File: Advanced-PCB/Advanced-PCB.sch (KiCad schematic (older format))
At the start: 150 parts, among them J1 USB_mini_micro_B, SW1 Esc, SW10 Win 1.25, SW11 2, SW12 W, SW13 S, SW14 X, SW15 Alt 1.25, SW16 3, SW17 E, SW18 D, SW19 C, SW2 Tab 1.50, SW20 4, SW21 R, SW22 F, SW23 V, SW24 5, SW25 T, SW26 G, SW27 B, SW28 Space 6.25, SW29 6, SW3 Caps 1.75, SW30 Y, SW31 H, SW32 N, SW33 7, SW34 U, SW35 J, SW36 M, SW37 8, SW38 I, SW39 K, SW4 Shift 2.25, SW40 ,, SW41 9, SW42 O, SW43 L, SW44 ., SW45 Alt 1.25, SW46 0, SW47 P, SW48 ;, SW49 /, SW5 Ctrl 1.25, SW50 Fn 1.25, SW51 -, SW52 [, SW53 ', SW54 Shift 1.75, SW55 Left Arrow, SW56 =, SW57 ], SW58 Enter 2.25, SW59 Up Arrow, SW6 1, SW60 Down Arrow, SW61 Back 2.00, SW62 \\ 1.50, SW63 Pg Up, SW64 Pg Down, SW65 Right Arrow, SW66 `, SW67 Del, SW7 Q, SW8 A, SW9 Z, U1 ATMEGA32U4, X1 16MHz

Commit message: Alternate Row 0
Alternate Row zero with 1u right side keys added.
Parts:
- added D? (x3): 1N4148W, Diode_SMD:D_SOD-123, symbol Device:D_Small
- added SW?: Fn 1.00, acheron_MXH:MX125H, symbol acheronSymbols:MXSwitch
- added SW?: Alt 1.00, acheron_MXH:MX125H, symbol acheronSymbols:MXSwitch
- added SW?: Ctrl 1.00, acheron_MXH:MX125H, symbol acheronSymbols:MXSwitch
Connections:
- wire segments 305 -> 315
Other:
- note added: "BOTTOM LAYOUT 1\n"
- note added: "BOTTOM LAYOUT 2\n\n"

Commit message: Layout Simplified
Layout Simplified by stacking switches unable to be used at same time because of different kb layouts. Right alt and fn with ctrl left down as seperate row.
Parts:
- removed D? (x2): 1N4148W, Diode_SMD:D_SOD-123, symbol Device:D_Small
- J1: symbol keyboard_parts:USB_mini_micro_B -> Advanced-PCB-rescue:USB_mini_micro_B-keyboard_parts
- SW1, SW10, SW11, SW12, SW13, SW14, SW15, SW16, SW17, SW18, SW19, SW2, SW20, SW21, SW22, SW23, SW24, SW25, SW26, SW27, SW28, SW29, SW3, SW30, SW31, SW32, SW33, SW34, SW35, SW36, SW37, SW38, SW39, SW4, SW40, SW41, SW42, SW43, SW44, SW45, SW46, SW47, SW48, SW49, SW5, SW50, SW51, SW52, SW53, SW54, SW55, SW56, SW57, SW58, SW59, SW6, SW60, SW61, SW62, SW63, SW64, SW65, SW66, SW67, SW7, SW8, SW9: symbol acheronSymbols:MXSwitch -> Advanced-PCB-rescue:MXSwitch-acheronSymbols
- SW68, SW69, SW70: renamed from SW?; footprint acheron_MXH:MX125H -> acheron_MXH:MX100H; symbol acheronSymbols:MXSwitch -> Advanced-PCB-rescue:MXSwitch-acheronSymbols
- SWPw1: symbol keyboard_parts:SW_PUSH -> Advanced-PCB-rescue:SW_PUSH-keyboard_parts
- U1: symbol keyboard_parts:ATMEGA32U4 -> Advanced-PCB-rescue:ATMEGA32U4-keyboard_parts
- X1: symbol keyboard_parts:XTAL_GND -> Advanced-PCB-rescue:XTAL_GND-keyboard_parts
- gave numbers to parts that had none: 1
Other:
- moved on the sheet: D70

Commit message: Rows And Columns Fixed
Fixed Issue to make all columns and rows linked properly
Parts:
- SW1, SW11, SW12, SW13, SW14, SW16, SW17, SW18, SW19, SW20, SW21, SW22, SW23, SW24, SW25, SW26, SW27, SW29, SW30, SW31, SW32, SW33, SW34, SW35, SW36, SW37, SW38, SW39, SW40, SW41, SW43, SW44, SW46, SW48, SW49, SW51, SW52, SW53, SW55, SW56, SW57, SW59, SW6, SW60, SW63, SW64, SW65, SW66, SW67, SW68, SW69, SW7, SW70, SW8, SW9: footprint acheron_MXH:MX100H -> acheron_MXA:MXA100
- SW10, SW15, SW45, SW5, SW50: footprint acheron_MXH:MX125H -> acheron_MXA:MXA125
- SW2, SW62: footprint acheron_MXH:MX150H -> acheron_MXA:MXA150
- SW28: footprint acheron_MXH:MX625HR -> acheron_MXA:MXA625R
- SW3, SW54: footprint acheron_MXH:MX175H -> acheron_MXA:MXA175
- SW4, SW58: footprint acheron_MXH:MX225HR -> acheron_MXA:MXA225R
- SW42: value O -> P; footprint acheron_MXH:MX100H -> acheron_MXA:MXA100
- SW47: value P -> O; footprint acheron_MXH:MX100H -> acheron_MXA:MXA100
- SW61: footprint acheron_MXH:MX200HR -> acheron_MXA:MXA200R
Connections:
- net Col1: now also U1.36 (PF7); no longer D1.1 (K), D10.1 (K), D11.1 (K), D12.1 (K), D13.1 (K), D14.1 (K), D15.1 (K), D16.1 (K), D17.1 (K), D18.1 (K), D19.1 (K), D2.1 (K), D20.1 (K), D21.1 (K), D22.1 (K), D23.1 (K), D24.1 (K), D25.1 (K), D26.1 (K), D27.1 (K), D28.1 (K), D29.1 (K), D3.1 (K), D30.1 (K), D31.1 (K), D32.1 (K), D33.1 (K), D34.1 (K), D35.1 (K), D36.1 (K), D37.1 (K), D38.1 (K), D39.1 (K), D4.1 (K), D40.1 (K), D41.1 (K), D42.1 (K), D43.1 (K), D44.1 (K), D45.1 (K), D46.1 (K), D47.1 (K), D48.1 (K), D49.1 (K), D5.1 (K), D50.1 (K), D51.1 (K), D52.1 (K), D53.1 (K), D54.1 (K), D55.1 (K), D56.1 (K), D57.1 (K), D58.1 (K), D59.1 (K), D6.1 (K), D60.1 (K), D61.1 (K), D62.1 (K), D63.1 (K), D64.1 (K), D65.1 (K), D66.1 (K), D67.1 (K), D7.1 (K), D70.1 (K), D8.1 (K), D9.1 (K), SW10.1 (Col), SW11.1 (Col), SW12.1 (Col), SW13.1 (Col), SW14.1 (Col), SW15.1 (Col), SW16.1 (Col), SW17.1 (Col), SW18.1 (Col), SW19.1 (Col), SW20.1 (Col), SW21.1 (Col), SW22.1 (Col), SW23.1 (Col), SW24.1 (Col), SW25.1 (Col), SW26.1 (Col), SW27.1 (Col), SW28.1 (Col), SW29.1 (Col), SW30.1 (Col), SW31.1 (Col), SW32.1 (Col), SW33.1 (Col), SW34.1 (Col), SW35.1 (Col), SW36.1 (Col), SW37.1 (Col), SW38.1 (Col), SW39.1 (Col), SW40.1 (Col), SW41.1 (Col), SW42.1 (Col), SW43.1 (Col), SW44.1 (Col), SW45.1 (Col), SW46.1 (Col), SW47.1 (Col), SW48.1 (Col), SW49.1 (Col), SW50.1 (Col), SW51.1 (Col), SW52.1 (Col), SW53.1 (Col), SW54.1 (Col), SW55.1 (Col), SW56.1 (Col), SW57.1 (Col), SW58.1 (Col), SW59.1 (Col), SW6.1 (Col), SW60.1 (Col), SW61.1 (Col), SW62.1 (Col), SW63.1 (Col), SW64.1 (Col), SW65.1 (Col), SW66.1 (Col), SW67.1 (Col), SW7.1 (Col), SW70.1 (Col), SW8.1 (Col), SW9.1 (Col), U1.38 (PF5), U1.39 (PF4), U1.40 (PF1), U1.41 (PF0)
- net Col10: now reaches U1.11 (PB3/MISO)
- net Col10: now also SW41.1 (Col), SW42.1 (Col), SW43.1 (Col), SW44.1 (Col), SW45.1 (Col), SW68.1 (Col)
- net Col11: now reaches U1.18 (PD0/INT0)
- net Col11: now also SW46.1 (Col), SW47.1 (Col), SW48.1 (Col), SW49.1 (Col), SW50.1 (Col), SW69.1 (Col)
- net Col12: now reaches U1.19 (PD1/INT1)
- net Col12: now also SW51.1 (Col), SW52.1 (Col), SW53.1 (Col), SW54.1 (Col), SW55.1 (Col), SW70.1 (Col)
- net Col13: now reaches U1.20 (PD2/RXD1)
- net Col13: now also SW56.1 (Col), SW57.1 (Col), SW58.1 (Col), SW59.1 (Col), SW60.1 (Col)
- net Col14: now reaches U1.21 (PD3/TXD1)
- net Col14: now also SW61.1 (Col), SW62.1 (Col), SW63.1 (Col), SW64.1 (Col), SW65.1 (Col)
- net Col15: now reaches U1.22 (PD5/XCK1)
- net Col15: now also SW66.1 (Col), SW67.1 (Col)
- net Col9: now reaches U1.25 (ICP1/PD4)
- net Col9: now also SW37.1 (Col), SW38.1 (Col), SW39.1 (Col), SW40.1 (Col)
- net Col8: now reaches U1.26 (T1/PD6)
- net Col8: now also SW33.1 (Col), SW34.1 (Col), SW35.1 (Col), SW36.1 (Col)
- net Col7: now reaches U1.27 (T0/PD7)
- net Col7: now also SW29.1 (Col), SW30.1 (Col), SW31.1 (Col), SW32.1 (Col)
- net Col6: now reaches U1.28 (PB4)
- net Col6: now also SW24.1 (Col), SW25.1 (Col), SW26.1 (Col), SW27.1 (Col), SW28.1 (Col)
- net Col5: now reaches U1.29 (PB5)
- net Col5: now also SW20.1 (Col), SW21.1 (Col), SW22.1 (Col), SW23.1 (Col)
- net Col4: now reaches U1.30 (PB6)
- net Col4: now also SW16.1 (Col), SW17.1 (Col), SW18.1 (Col), SW19.1 (Col)
- net Col3: now reaches U1.31 (PC6)
- net Col3: now also SW11.1 (Col), SW12.1 (Col), SW13.1 (Col), SW14.1 (Col), SW15.1 (Col)
- net Col2: now reaches U1.32 (PC7)
- net Col2: now also SW10.1 (Col), SW6.1 (Col), SW7.1 (Col), SW8.1 (Col), SW9.1 (Col)
- net Row4: now reaches U1.37 (PF6)
- net Row4: now also D1.1 (K), D11.1 (K), D16.1 (K), D20.1 (K), D24.1 (K), D29.1 (K), D33.1 (K), D37.1 (K), D41.1 (K), D46.1 (K), D51.1 (K), D56.1 (K), D6.1 (K), D61.1 (K), D66.1 (K)
- net at D45.2 (A), SW45.2 (Row): now also SW68.2 (Row)
- net at D50.2 (A), SW50.2 (Row): now also SW69.2 (Row)
- new net Row0: D10.1 (K), D15.1 (K), D28.1 (K), D45.1 (K), D5.1 (K), D50.1 (K), D55.1 (K), D60.1 (K), D65.1 (K), D70.1 (K), U1.41 (PF0)
- new net Row1: D14.1 (K), D19.1 (K), D23.1 (K), D27.1 (K), D32.1 (K), D36.1 (K), D4.1 (K), D40.1 (K), D44.1 (K), D49.1 (K), D54.1 (K), D59.1 (K), D64.1 (K), D9.1 (K), U1.40 (PF1)
- new net Row2: D13.1 (K), D18.1 (K), D22.1 (K), D26.1 (K), D3.1 (K), D31.1 (K), D35.1 (K), D39.1 (K), D43.1 (K), D48.1 (K), D53.1 (K), D58.1 (K), D63.1 (K), D8.1 (K), U1.39 (PF4)
- new net Row3: D12.1 (K), D17.1 (K), D2.1 (K), D21.1 (K), D25.1 (K), D30.1 (K), D34.1 (K), D38.1 (K), D42.1 (K), D47.1 (K), D52.1 (K), D57.1 (K), D62.1 (K), D67.1 (K), D7.1 (K), U1.38 (PF5)
- no-connect marks 22 -> 6
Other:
- moved on the sheet: D45, D50

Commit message: Mid Routing
In the Middle of Routing. All of tracing between initial components done. Switches still need to be traced and connected.
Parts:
- J1: symbol Advanced-PCB-rescue:USB_mini_micro_B-keyboard_parts -> Advanced-PCB-rescue:USB_mini_micro_B-keyboard_parts-Advanced-PCB-rescue
- SW1, SW10, SW11, SW12, SW13, SW14, SW15, SW16, SW17, SW18, SW19, SW2, SW20, SW21, SW22, SW23, SW24, SW25, SW26, SW27, SW28, SW29, SW3, SW30, SW31, SW32, SW33, SW34, SW35, SW36, SW37, SW38, SW39, SW4, SW40, SW41, SW42, SW43, SW44, SW45, SW46, SW47, SW48, SW49, SW5, SW50, SW51, SW52, SW53, SW54, SW55, SW56, SW57, SW58, SW59, SW6, SW60, SW61, SW62, SW63, SW64, SW65, SW66, SW67, SW68, SW69, SW7, SW70, SW8, SW9: symbol Advanced-PCB-rescue:MXSwitch-acheronSymbols -> Advanced-PCB-rescue:MXSwitch-acheronSymbols-Advanced-PCB-rescue
- SWPw1: symbol Advanced-PCB-rescue:SW_PUSH-keyboard_parts -> Advanced-PCB-rescue:SW_PUSH-keyboard_parts-Advanced-PCB-rescue
- U1: symbol Advanced-PCB-rescue:ATMEGA32U4-keyboard_parts -> Advanced-PCB-rescue:ATMEGA32U4-keyboard_parts-Advanced-PCB-rescue
- X1: value 16MHz -> XTAL_GND; footprint Crystal:Crystal_SMD_SeikoEpson_TSX3225-4Pin_3.2x2.5mm_HandSoldering -> kicad-library-master:crystal_FA238-TSX3225; symbol Advanced-PCB-rescue:XTAL_GND-keyboard_parts -> Advanced-PCB-rescue:XTAL_GND-keyboard_parts-Advanced-PCB-rescue
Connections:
- net +5V renamed GND

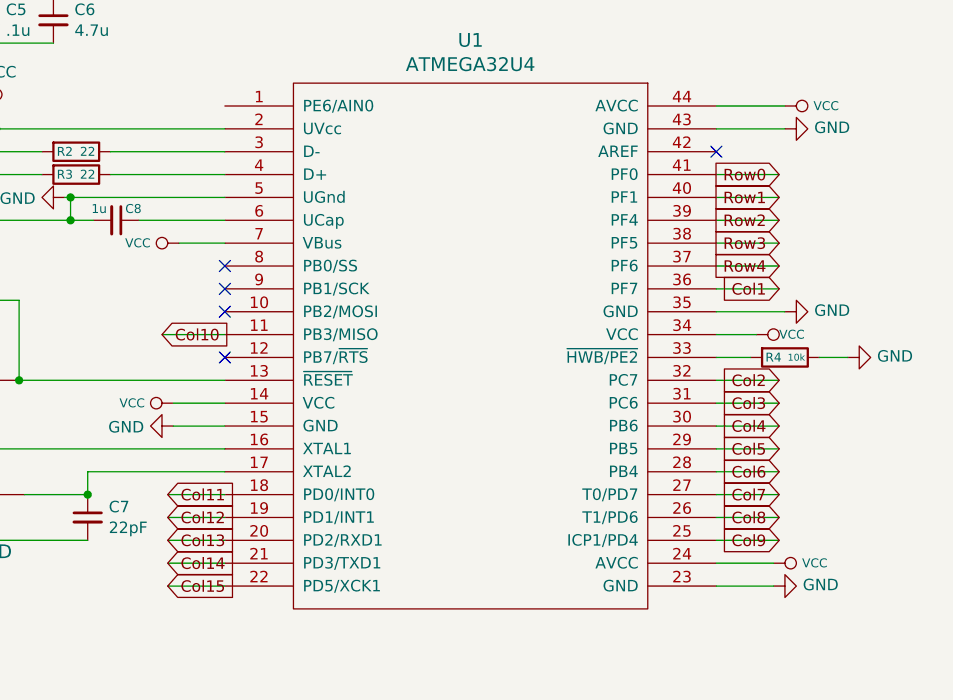
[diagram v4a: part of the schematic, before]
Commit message: Traces Continued
Continued Tracing All Rows and Half Columns completed.
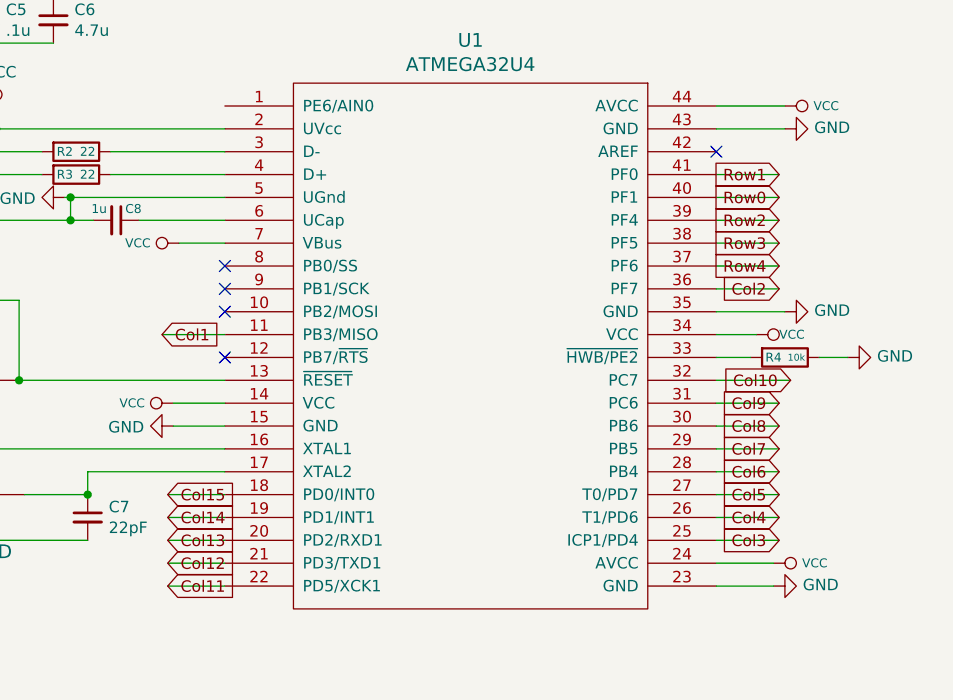
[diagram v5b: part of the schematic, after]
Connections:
- net Col1: now also U1.11 (PB3/MISO); no longer U1.36 (PF7)
- net Col10: now also U1.32 (PC7); no longer U1.11 (PB3/MISO)
- net Col11: now also U1.22 (PD5/XCK1); no longer U1.18 (PD0/INT0)
- net Col12: now also U1.21 (PD3/TXD1); no longer U1.19 (PD1/INT1)
- net Col14: now also U1.19 (PD1/INT1); no longer U1.21 (PD3/TXD1)
- net Col15: now also U1.18 (PD0/INT0); no longer U1.22 (PD5/XCK1)
- net Col2: now also U1.36 (PF7); no longer U1.32 (PC7)
- net Col3: now also U1.25 (ICP1/PD4); no longer U1.31 (PC6)
- net Col4: now also U1.26 (T1/PD6); no longer U1.30 (PB6)
- net Col5: now also U1.27 (T0/PD7); no longer U1.29 (PB5)
- net Col7: now also U1.29 (PB5); no longer U1.27 (T0/PD7)
- net Col8: now also U1.30 (PB6); no longer U1.26 (T1/PD6)
- net Col9: now also U1.31 (PC6); no longer U1.25 (ICP1/PD4)
- net Row0: now also U1.40 (PF1); no longer U1.41 (PF0)
- net Row1: now also U1.41 (PF0); no longer U1.40 (PF1)
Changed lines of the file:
@@
 	0    -1   -1   0
-$EndComp
-$Comp
-L Device:R R4
-U 1 1 5E649C11
-P 5575 14375
-F 0 "R4" V 5575 14325 39  0000 C CNN
-F 1 "10k" V 5575 14425 30  0000 C CNN
-F 2 "Resistor_SMD:R_0805_2012Metric_Pad1.15x1.40mm_HandSolder" V 5505 14375 50  0001 C CNN
-F 3 "~" H 5575 14375 50  0001 C CNN
-	1    5575 14375
-	0    1    1    0
 $EndComp
 Wire Wire Line
@@
 NoConn ~ 5275 13475
 Text GLabel 5550 13575 0    50   Input ~ 0
-Row0
-Text GLabel 5550 13675 0    50   Input ~ 0
 Row1
-Text GLabel 5550 13775 0    50   Input ~ 0
-Row2
-Text GLabel 5550 13875 0    50   Input ~ 0
-Row3
-Text GLabel 5550 13975 0    50   Input ~ 0
-Row4
-Wire Wire Line
-	5275 13575 5550 13575
-Wire Wire Line
-	5275 13675 5550 13675
-Wire Wire Line
-	5275 13775 5550 13775
-Wire Wire Line
-	5275 13875 5550 13875
-Wire Wire Line
-	5275 13975 5550 13975
-Text GLabel 5550 14075 0    50   Input ~ 0
-Col1
-Text GLabel 5550 14475 0    50   Input ~ 0
-Col2
-Text GLabel 5550 14575 0    50   Input ~ 0
+Wire Wire Line
+	3125 14275 2850 14275
+Text GLabel 5550 15175 0    50   Input ~ 0
 Col3
-Text GLabel 5550 14675 0    50   Input ~ 0
+Text GLabel 5550 15075 0    50   Input ~ 0
 Col4
-Text GLabel 5550 14775 0    50   Input ~ 0
+Text GLabel 5550 14975 0    50   Input ~ 0
 Col5
 Text GLabel 5550 14875 0    50   Input ~ 0
 Col6
-Text GLabel 5550 14975 0    50   Input ~ 0
+Text GLabel 5550 14575 0    50   Input ~ 0
+Col9
+Text GLabel 5550 14675 0    50   Input ~ 0
+Col8
+Text GLabel 5550 14775 0    50   Input ~ 0
 Col7
-Text GLabel 5550 15075 0    50   Input ~ 0
-Col8
-Text GLabel 5550 15175 0    50   Input ~ 0
-Col9
-Wire Wire Line
-	5275 14075 5550 14075
 $Comp
 L Advanced-PCB-rescue:ATMEGA32U4-keyboard_parts-Advanced-PCB-rescue U1
@@
 $EndComp
 Wire Wire Line
-	5275 14475 5550 14475
+	5275 15175 5550 15175
+Wire Wire Line
+	5275 15075 5550 15075
+Wire Wire Line
+	5275 14975 5550 14975
+Wire Wire Line
+	5275 14875 5550 14875
 Wire Wire Line
 	5275 14575 5550 14575
@@
 Wire Wire Line
 	5275 14775 5550 14775
-Wire Wire Line
-	5275 14875 5550 14875
-Wire Wire Line
-	5275 14975 5550 14975
-Wire Wire Line
-	5275 15075 5550 15075
-Wire Wire Line
-	5275 15175 5550 15175
-Text GLabel 2850 14275 2    50   Input ~ 0
+Text GLabel 5600 14475 0    50   Input ~ 0
 Col10
-Wire Wire Line
-	2850 14275 3125 14275
 Text GLabel 2875 14975 2    50   Input ~ 0
-Col11
+Col15
 Text GLabel 2875 15075 2    50   Input ~ 0
-Col12
+Col14
 Text GLabel 2875 15175 2    50   Input ~ 0
 Col13
 Text GLabel 2875 15275 2    50   Input ~ 0
-Col14
+Col12
 Text GLabel 2875 15375 2    50   Input ~ 0
-Col15
+Col11
 Wire Wire Line
 	2875 15375 3125 15375
@@
 $EndComp
 $Comp
+L power:GND #PWR0109
+U 1 1 5EFF7077
+P 5575 13375
+F 0 "#PWR0109" H 5575 13125 50  0001 C CNN
+F 1 "GND" V 5580 13247 50  0000 R CNN
+F 2 "" H 5575 13375 50  0001 C CNN
+F 3 "" H 5575 13375 50  0001 C CNN
+	1    5575 13375
+	0    -1   -1   0
+$EndComp
+$Comp
+L Device:R R1
+U 1 1 5E67690A
+P 1925 14125
+F 0 "R1" V 1850 14125 50  0000 C CNN
+F 1 "10k" V 1925 14125 50  0000 C CNN
+F 2 "Resistor_SMD:R_0805_2012Metric_Pad1.15x1.40mm_HandSolder" V 1855 14125 50  0001 C CNN
+F 3 "~" H 1925 14125 50  0001 C CNN
+	1    1925 14125
+	0    1    1    0
+$EndComp
+Wire Wire Line
+	1500 14125 1775 14125
+Wire Wire Line
+	5275 14475 5600 14475
+$Comp
+L Device:R R4
+U 1 1 5E649C11
+P 5575 14375
+F 0 "R4" V 5575 14325 39  0000 C CNN
+F 1 "10k" V 5575 14425 30  0000 C CNN
+F 2 "Resistor_SMD:R_0805_2012Metric_Pad1.15x1.40mm_HandSolder" V 5505 14375 50  0001 C CNN
+F 3 "~" H 5575 14375 50  0001 C CNN
+	1    5575 14375
+	0    1    1    0
+$EndComp
+Text GLabel 5550 14075 0    50   Input ~ 0
+Col2
+Wire Wire Line
+	5275 14075 5550 14075
+$Comp
 L power:GND #PWR0108
 U 1 1 5EFB7B99
@@
 	0    -1   -1   0
 $EndComp
-$Comp
-L power:GND #PWR0109
-U 1 1 5EFF7077
-P 5575 13375
-F 0 "#PWR0109" H 5575 13125 50  0001 C CNN
-F 1 "GND" V 5580 13247 50  0000 R CNN
-F 2 "" H 5575 13375 50  0001 C CNN
-F 3 "" H 5575 13375 50  0001 C CNN
-	1    5575 13375
-	0    -1   -1   0
-$EndComp
-$Comp
-L Device:R R1
-U 1 1 5E67690A
-P 1925 14125
-F 0 "R1" V 1850 14125 50  0000 C CNN
-F 1 "10k" V 1925 14125 50  0000 C CNN
-F 2 "Resistor_SMD:R_0805_2012Metric_Pad1.15x1.40mm_HandSolder" V 1855 14125 50  0001 C CNN
-F 3 "~" H 1925 14125 50  0001 C CNN
-	1    1925 14125
-	0    1    1    0
-$EndComp
-Wire Wire Line
-	1500 14125 1775 14125
+Text GLabel 2850 14275 2    50   Input ~ 0
+Col1
+Wire Wire Line
+	5275 13975 5550 13975
+Wire Wire Line
+	5275 13875 5550 13875
+Wire Wire Line
+	5275 13775 5550 13775
+Wire Wire Line
+	5275 13675 5550 13675
+Text GLabel 5550 13975 0    50   Input ~ 0
+Row4
+Text GLabel 5550 13875 0    50   Input ~ 0
+Row3
+Text GLabel 5550 13775 0    50   Input ~ 0
+Row2
+Text GLabel 5550 13675 0    50   Input ~ 0
+Row0
+Wire Wire Line
+	5275 13575 5550 13575
 $EndSCHEMATC

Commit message: PCB-Rerouted
Correctly Rerouted and except of errors except for with layer keys.
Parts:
- SW45, SW50: footprint acheron_MXA:MXA125 -> acheron_MX:MX125
- SW68, SW69: footprint acheron_MXA:MXA100 -> acheron_MX:MX100
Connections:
- net Col1: now also U1.41 (PF0); no longer U1.11 (PB3/MISO)
- net Col10: now also U1.30 (PB6); no longer U1.32 (PC7)
- net Col11: now also U1.25 (ICP1/PD4); no longer U1.22 (PD5/XCK1)
- net Col12: now also U1.26 (T1/PD6); no longer U1.21 (PD3/TXD1)
- net Col13: now also U1.27 (T0/PD7); no longer U1.20 (PD2/RXD1)
- net Col14: now also U1.28 (PB4); no longer U1.19 (PD1/INT1)
- net Col15: now also U1.29 (PB5); no longer U1.18 (PD0/INT0)
- net Col2: now also U1.40 (PF1); no longer U1.36 (PF7)
- net Col3: now also U1.39 (PF4); no longer U1.25 (ICP1/PD4)
- net Col4: now also U1.38 (PF5); no longer U1.26 (T1/PD6)
- net Col5: now also U1.37 (PF6); no longer U1.27 (T0/PD7)
- net Col6: now also U1.11 (PB3/MISO); no longer U1.28 (PB4)
- net Col7: now also U1.36 (PF7); no longer U1.29 (PB5)
- net Col8: now also U1.32 (PC7); no longer U1.30 (PB6)
- net Row0: now also U1.42 (AREF); no longer U1.40 (PF1)
- net Row1: now also U1.22 (PD5/XCK1); no longer U1.41 (PF0)
- net Row2: now also U1.21 (PD3/TXD1); no longer U1.39 (PF4)
- net Row3: now also U1.20 (PD2/RXD1); no longer U1.38 (PF5)
- net Row4: now also U1.19 (PD1/INT1); no longer U1.37 (PF6)
- net at D46.2 (A): now also SW46.2 (Row)
- no-connect marks 6 -> 7
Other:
- moved on the sheet: D46
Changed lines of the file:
@@
 	10900 1000 10900 1250
 Connection ~ 9700 1775
-Connection ~ 10050 1000
-Wire Wire Line
-	10050 1000 10050 1275
 $Comp
 L Device:D_Small D51
@@
 L Device:D_Small D46
 U 1 1 5E834C3E
-P 10050 1375
-F 0 "D46" V 10125 1425 50  0000 L CNN
-F 1 "1N4148W" V 9925 1250 50  0000 L CNN
-F 2 "Diode_SMD:D_SOD-123" V 10050 1375 50  0001 C CNN
-F 3 "~" V 10050 1375 50  0001 C CNN
-	1    10050 1375
+P 10050 1325
+F 0 "D46" V 10125 1375 50  0000 L CNN
+F 1 "1N4148W" V 9925 1200 50  0000 L CNN
+F 2 "Diode_SMD:D_SOD-123" V 10050 1325 50  0001 C CNN
+F 3 "~" V 10050 1325 50  0001 C CNN
+	1    10050 1325
 	0    1    1    0
 $EndComp
@@
 F 0 "SW50" H 10250 7000 50  0000 L CNN
 F 1 "Fn 1.25" H 10350 6925 59  0000 C CNN
-F 2 "acheron_MXA:MXA125" H 10050 6625 50  0001 C CNN
+F 2 "acheron_MX:MX125" H 10050 6625 50  0001 C CNN
 F 3 "" H 10050 6625 50  0001 C CNN
 	1    10050 6625
@@
 F 0 "SW69" H 9950 6275 50  0000 L CNN
 F 1 "Fn 1.00" H 10025 6350 59  0000 C CNN
-F 2 "acheron_MXA:MXA100" H 10125 6675 50  0001 C CNN
+F 2 "acheron_MX:MX100" H 10125 6675 50  0001 C CNN
 F 3 "" H 10125 6675 50  0001 C CNN
 	1    10125 6675
@@
 F 0 "SW45" H 9350 7000 50  0000 L CNN
 F 1 "Alt 1.25" H 9450 6925 59  0000 C CNN
-F 2 "acheron_MXA:MXA125" H 9200 6625 50  0001 C CNN
+F 2 "acheron_MX:MX125" H 9200 6625 50  0001 C CNN
 F 3 "" H 9200 6625 50  0001 C CNN
 	1    9200 6625
@@
 F 0 "SW68" H 9150 6350 50  0000 L CNN
 F 1 "Alt 1.00" H 9250 6275 59  0000 C CNN
-F 2 "acheron_MXA:MXA100" H 9250 6650 50  0001 C CNN
+F 2 "acheron_MX:MX100" H 9250 6650 50  0001 C CNN
 F 3 "" H 9250 6650 50  0001 C CNN
 	1    9250 6650
@@
 	10125 6275 10050 6275
 NoConn ~ 5275 13475
-Text GLabel 5550 13575 0    50   Input ~ 0
+Text GLabel 2850 15375 2    50   Input ~ 0
 Row1
 Wire Wire Line
-	3125 14275 2850 14275
-Text GLabel 5550 15175 0    50   Input ~ 0
+	5275 13575 5550 13575
+Text GLabel 5550 13775 0    50   Input ~ 0
 Col3
-Text GLabel 5550 15075 0    50   Input ~ 0
+Text GLabel 5550 13875 0    50   Input ~ 0
 Col4
-Text GLabel 5550 14975 0    50   Input ~ 0
+Text GLabel 5550 13975 0    50   Input ~ 0
 Col5
-Text GLabel 5550 14875 0    50   Input ~ 0
+Text GLabel 2850 14275 2    50   Input ~ 0
 Col6
 Text GLabel 5550 14575 0    50   Input ~ 0
 Col9
-Text GLabel 5550 14675 0    50   Input ~ 0
+Text GLabel 5550 14475 0    50   Input ~ 0
 Col8
-Text GLabel 5550 14775 0    50   Input ~ 0
+Text GLabel 5550 14075 0    50   Input ~ 0
 Col7
 $Comp
@@
 $EndComp
 Wire Wire Line
-	5275 15175 5550 15175
-Wire Wire Line
-	5275 15075 5550 15075
-Wire Wire Line
-	5275 14975 5550 14975
-Wire Wire Line
-	5275 14875 5550 14875
+	5275 13775 5550 13775
+Wire Wire Line
+	5275 13875 5550 13875
+Wire Wire Line
+	5275 13975 5550 13975
+Wire Wire Line
+	3125 14275 2850 14275
 Wire Wire Line
 	5275 14575 5550 14575
 Wire Wire Line
-	5275 14675 5550 14675
-Wire Wire Line
-	5275 14775 5550 14775
-Text GLabel 5600 14475 0    50   Input ~ 0
+	5275 14475 5550 14475
+Wire Wire Line
+	5275 14075 5550 14075
+Text GLabel 5600 14675 0    50   Input ~ 0
 Col10
-Text GLabel 2875 14975 2    50   Input ~ 0
+Text GLabel 5525 14775 0    50   Input ~ 0
 Col15
-Text GLabel 2875 15075 2    50   Input ~ 0
+Text GLabel 5525 14875 0    50   Input ~ 0
 Col14
-Text GLabel 2875 15175 2    50   Input ~ 0
+Text GLabel 5525 14975 0    50   Input ~ 0
 Col13
-Text GLabel 2875 15275 2    50   Input ~ 0
+Text GLabel 5525 15075 0    50   Input ~ 0
 Col12
-Text GLabel 2875 15375 2    50   Input ~ 0
-Col11
-Wire Wire Line
-	2875 15375 3125 15375
-Wire Wire Line
-	2875 15275 3125 15275
-Wire Wire Line
-	2875 15175 3125 15175
-Wire Wire Line
-	2875 15075 3125 15075
-Wire Wire Line
-	2875 14975 3125 14975
+Wire Wire Line
+	5525 15075 5275 15075
+Wire Wire Line
+	5525 14975 5275 14975
+Wire Wire Line
+	5525 14875 5275 14875
+Wire Wire Line
+	5525 14775 5275 14775
 Connection ~ 13050 1775
 Wire Wire Line
@@
 Wire Wire Line
 	9700 825  9700 1775
-Wire Wire Line
-	9200 1000 10050 1000
 Connection ~ 10550 1800
 Wire Wire Line
 	10550 825  10550 1800
-Wire Wire Line
-	10050 1000 10900 1000
 Wire Wire Line
 	11350 825  11350 1775
@@
 	1500 14125 1775 14125
 Wire Wire Line
-	5275 14475 5600 14475
+	5275 14675 5600 14675
 $Comp
 L Device:R R4
@@
 	0    1    1    0
 $EndComp
-Text GLabel 5550 14075 0    50   Input ~ 0
+Text GLabel 5550 13675 0    50   Input ~ 0
 Col2
 Wire Wire Line
-	5275 14075 5550 14075
+	5275 13675 5550 13675
 $Comp
 L power:GND #PWR0108
@@
 	0    -1   -1   0
 $EndComp
-Text GLabel 2850 14275 2    50   Input ~ 0
+Text GLabel 5550 13575 0    50   Input ~ 0
 Col1
 Wire Wire Line
-	5275 13975 5550 13975
-Wire Wire Line
-	5275 13875 5550 13875
-Wire Wire Line
-	5275 13775 5550 13775
-Wire Wire Line
-	5275 13675 5550 13675
-Text GLabel 5550 13975 0    50   Input ~ 0
+	3125 15075 2850 15075
+Wire Wire Line
+	3125 15175 2850 15175
+Wire Wire Line
+	3125 15275 2850 15275
+Text GLabel 2850 15075 2    50   Input ~ 0
 Row4
-Text GLabel 5550 13875 0    50   Input ~ 0
+Text GLabel 2850 15175 2    50   Input ~ 0
 Row3
-Text GLabel 5550 13775 0    50   Input ~ 0
+Text GLabel 2850 15275 2    50   Input ~ 0
 Row2
-Text GLabel 5550 13675 0    50   Input ~ 0
+Wire Wire Line
+	3125 15375 2850 15375
+Wire Wire Line
+	9200 1000 10050 1000
+Wire Wire Line
+	10050 1225 10050 1000
+Connection ~ 10050 1000
+Wire Wire Line
+	10050 1000 10900 1000
+Wire Wire Line
+	5275 13475 5550 13475
+Text GLabel 5550 13475 0    50   Input ~ 0
 Row0
 Wire Wire Line
-	5275 13575 5550 13575
+	5525 15175 5275 15175
+Text GLabel 5525 15175 0    50   Input ~ 0
+Col11
+NoConn ~ 3125 14975
 $EndSCHEMATC
